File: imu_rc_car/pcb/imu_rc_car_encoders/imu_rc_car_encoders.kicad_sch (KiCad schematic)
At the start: 24 parts, among them J1 Conn_01x04_Socket, U2 LMV393, U3 ITR9608-F, U4 ITR9608-F

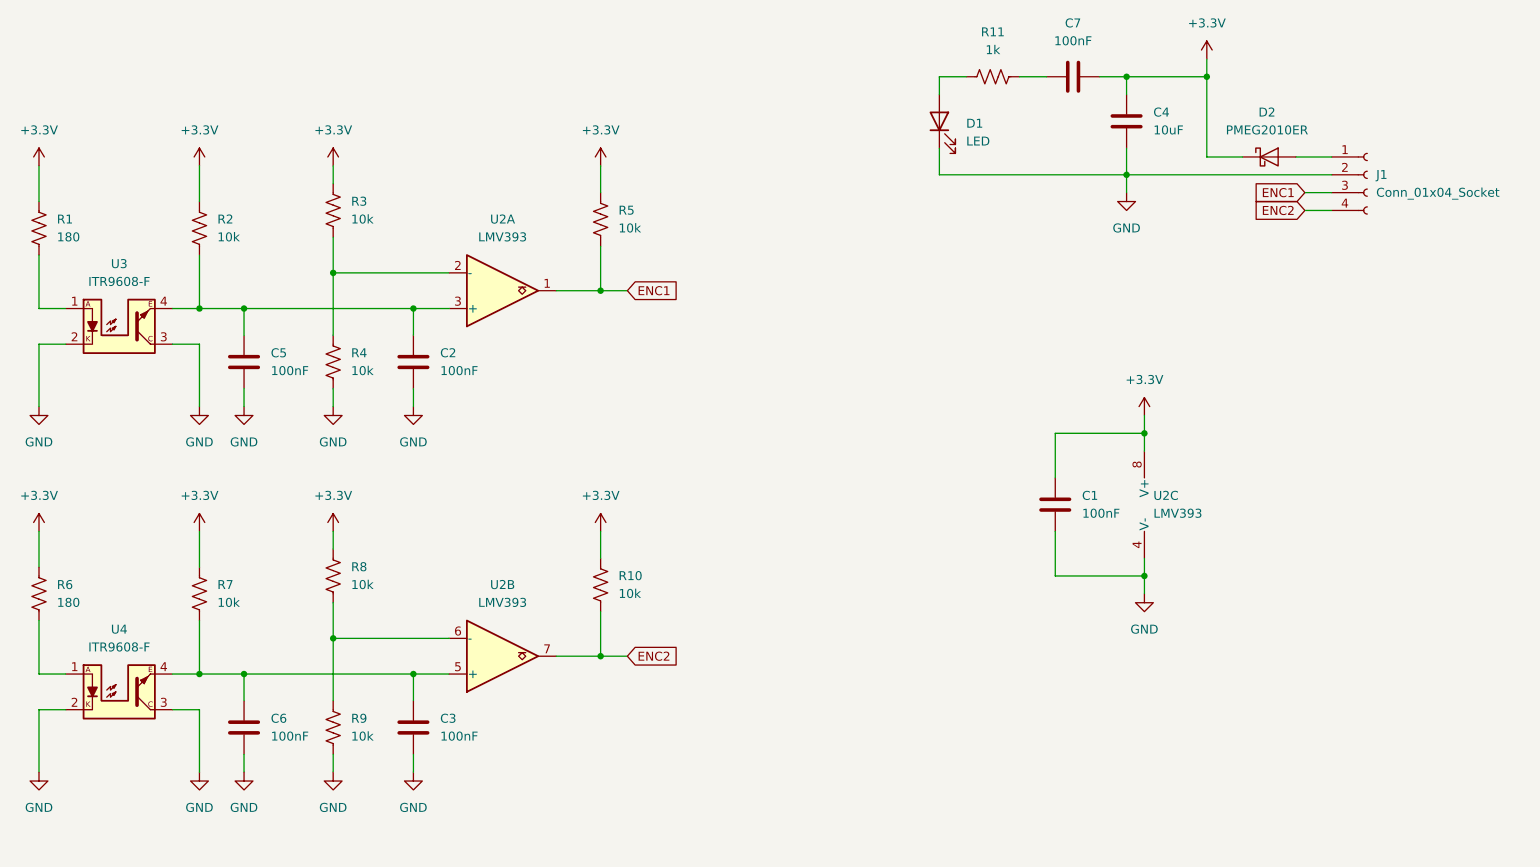
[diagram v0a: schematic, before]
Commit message: commit #17
IR Speed Encoder board v1.0
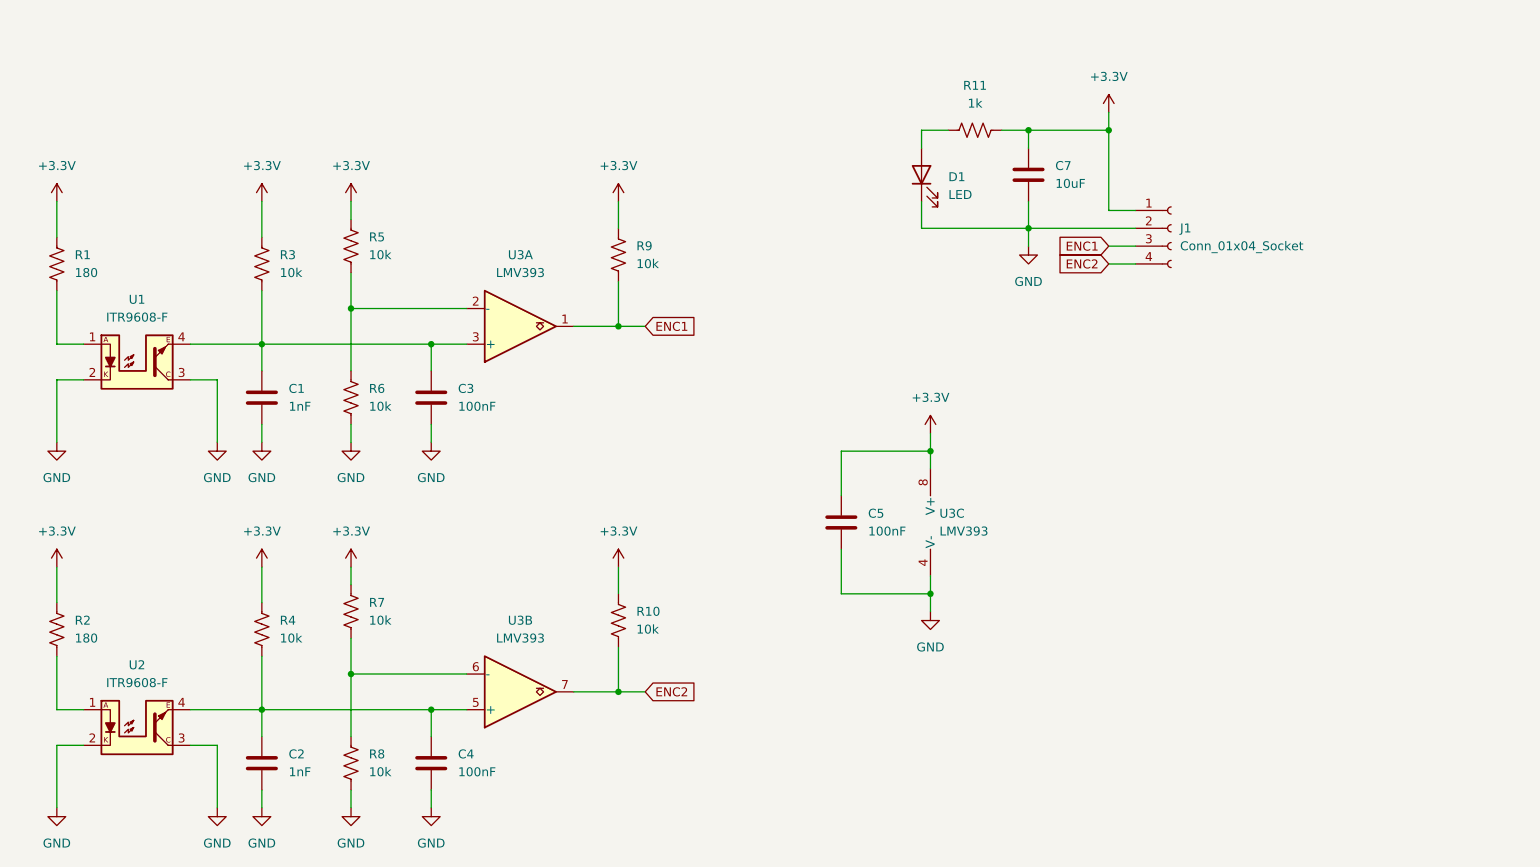
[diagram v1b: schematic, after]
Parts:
- removed C6: 100nF, Capacitor_SMD:C_0805_2012Metric, symbol Device:C
- removed D2: PMEG2010ER, Diode_SMD:Nexperia_CFP3_SOD-123W, symbol Diode:PMEG2010ER
- removed U2: LMV393, Package_SO:SOIC-8_3.9x4.9mm_P1.27mm, symbol Comparator:LMV393
- removed U3, U4: ITR9608-F, OptoDevice:Everlight_ITR9608-F, symbol Sensor_Proximity:ITR9608-F
- added U1, U2: ITR9608-F, OptoDevice:Everlight_ITR9608-F, symbol Sensor_Proximity:ITR9608-F
- added U3: LMV393, Package_SO:SOIC-8_3.9x4.9mm_P1.27mm, symbol Comparator:LMV393
- C1, C2: value 100nF -> 1nF
- C4: value 10uF -> 100nF
- C7: value 100nF -> 10uF
- J1: footprint Connector_JST:JST_PH_S4B-PH-K_1x04_P2.00mm_Horizontal -> Connector_JST:JST_PH_S4B-PH-SM4-TB_1x04-1MP_P2.00mm_Horizontal
- R2: value 10k -> 180
- R6: value 180 -> 10k
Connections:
- net +3.3V: now also C5.1, C7.1, J1.1 (Pin_1), R11.2, R4.1, R9.1, U3.8 (V+); no longer C1.1, C4.1, C7.2, R6.1, R8.1
- net ENC1: now also R9.2, U3.1; no longer R5.2
- net ENC2: now also U3.7
- net GND: now also C7.2, R6.2, R8.2, U1.2, U1.3, U2.2, U2.3, U3.4 (V-); no longer R4.2, R9.2
- net at R1.2: now also U1.1
- net at C3.1: now also C1.1, R3.2, U1.4, U3.3 (+); no longer R7.2
- new net: R2.2, U2.1
- new net: R5.2, R6.1, U3.2 (-)
- new net: C2.1, C4.1, R4.2, U2.4, U3.5 (+)
- new net: R7.2, R8.1, U3.6 (-)
